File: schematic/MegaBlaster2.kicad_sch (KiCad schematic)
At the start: 119 parts, among them J1 USB_B, J2 SWD, J3 Micro_SD_Card, J4 AudioJack3, J5 DAC_Enable, SW2 SW_Push_Dual, SW3 SW_Push_Dual, SW4 SW_Push_Dual, SW5 SW_Push_Dual, SW6 SW_Push_Dual, SW7 SW_Push_Dual, U1 ATSAMD51J19A-A, U10 TPA6111A2DR, U11 YM2151, U2 LM2733XMF, U3 LD1117S33TR_SOT223, U4 LD1117S50TR_SOT223, U5 W25Q32JVSS, U6 Si5351A-B-GT, U7 TL074, U8 YM3012, U9 MCP6004, Y1 32.768KHz, Y2 25MHz

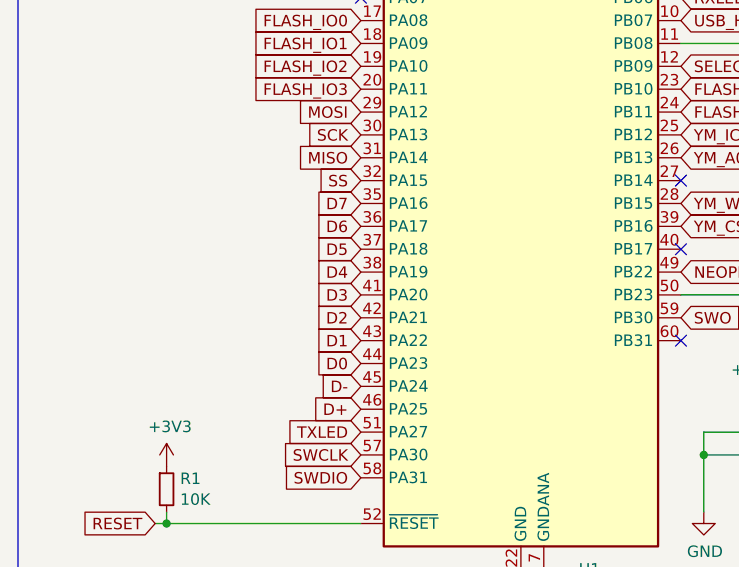
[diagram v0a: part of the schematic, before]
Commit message: PCB first pass
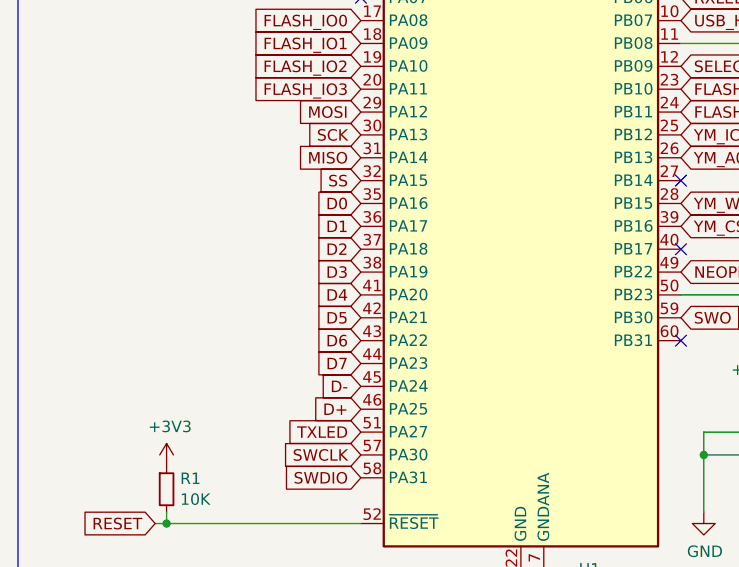
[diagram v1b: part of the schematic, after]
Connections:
- net D0: now also U1.35 (PA16); no longer U1.44 (PA23)
- net D1: now also U1.36 (PA17); no longer U1.43 (PA22)
- net D2: now also U1.37 (PA18); no longer U1.42 (PA21)
- net D3: now also U1.38 (PA19); no longer U1.41 (PA20)
- net D4: now also U1.41 (PA20); no longer U1.38 (PA19)
- net D5: now also U1.42 (PA21); no longer U1.37 (PA18)
- net D6: now also U1.43 (PA22); no longer U1.36 (PA17)
- net D7: now also U1.44 (PA23); no longer U1.35 (PA16)
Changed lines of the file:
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@@
     (effects (font (size 1.27 1.27)) (justify left bottom))
   )
-  (global_label "D7" (shape input) (at 52.07 87.63 180) (fields_autoplaced)
-    (effects (font (size 1.27 1.27)) (justify right))
-    (property "Intersheet References" "${INTERSHEET_REFS}" (id 0) (at 0 0 0)
+  (global_label "D7" (shape input) (at 52.07 105.41 180) (fields_autoplaced)
+    (effects (font (size 1.27 1.27)) (justify right))
+    (property "Intersheet References" "${INTERSHEET_REFS}" (id 0) (at 0 193.04 0)
       (effects (font (size 1.27 1.27)) hide)
     )
@@
     )
   )
-  (global_label "D4" (shape input) (at 52.07 95.25 180) (fields_autoplaced)
-    (effects (font (size 1.27 1.27)) (justify right))
-    (property "Intersheet References" "${INTERSHEET_REFS}" (id 0) (at 0 0 0)
+  (global_label "D4" (shape input) (at 52.07 97.79 180) (fields_autoplaced)
+    (effects (font (size 1.27 1.27)) (justify right))
+    (property "Intersheet References" "${INTERSHEET_REFS}" (id 0) (at 0 193.04 0)
       (effects (font (size 1.27 1.27)) hide)
     )
@@
     )
   )
-  (global_label "D2" (shape input) (at 52.07 100.33 180) (fields_autoplaced)
-    (effects (font (size 1.27 1.27)) (justify right))
-    (property "Intersheet References" "${INTERSHEET_REFS}" (id 0) (at 0 0 0)
+  (global_label "D2" (shape input) (at 52.07 92.71 180) (fields_autoplaced)
+    (effects (font (size 1.27 1.27)) (justify right))
+    (property "Intersheet References" "${INTERSHEET_REFS}" (id 0) (at 0 193.04 0)
       (effects (font (size 1.27 1.27)) hide)
     )
@@
     )
   )
-  (global_label "D5" (shape input) (at 52.07 92.71 180) (fields_autoplaced)
-    (effects (font (size 1.27 1.27)) (justify right))
-    (property "Intersheet References" "${INTERSHEET_REFS}" (id 0) (at 0 0 0)
+  (global_label "D5" (shape input) (at 52.07 100.33 180) (fields_autoplaced)
+    (effects (font (size 1.27 1.27)) (justify right))
+    (property "Intersheet References" "${INTERSHEET_REFS}" (id 0) (at 0 193.04 0)
       (effects (font (size 1.27 1.27)) hide)
     )
@@
     )
   )
-  (global_label "D3" (shape input) (at 52.07 97.79 180) (fields_autoplaced)
-    (effects (font (size 1.27 1.27)) (justify right))
-    (property "Intersheet References" "${INTERSHEET_REFS}" (id 0) (at 0 0 0)
+  (global_label "D3" (shape input) (at 52.07 95.25 180) (fields_autoplaced)
+    (effects (font (size 1.27 1.27)) (justify right))
+    (property "Intersheet References" "${INTERSHEET_REFS}" (id 0) (at 0 193.04 0)
       (effects (font (size 1.27 1.27)) hide)
     )
@@
     )
   )
-  (global_label "D6" (shape input) (at 52.07 90.17 180) (fields_autoplaced)
-    (effects (font (size 1.27 1.27)) (justify right))
-    (property "Intersheet References" "${INTERSHEET_REFS}" (id 0) (at 0 0 0)
-      (effects (font (size 1.27 1.27)) hide)
-    )
-  )
-  (global_label "D0" (shape input) (at 52.07 105.41 180) (fields_autoplaced)
-    (effects (font (size 1.27 1.27)) (justify right))
-    (property "Intersheet References" "${INTERSHEET_REFS}" (id 0) (at 0 0 0)
+  (global_label "D6" (shape input) (at 52.07 102.87 180) (fields_autoplaced)
+    (effects (font (size 1.27 1.27)) (justify right))
+    (property "Intersheet References" "${INTERSHEET_REFS}" (id 0) (at 0 193.04 0)
+      (effects (font (size 1.27 1.27)) hide)
+    )
+  )
+  (global_label "D0" (shape input) (at 52.07 87.63 180) (fields_autoplaced)
+    (effects (font (size 1.27 1.27)) (justify right))
+    (property "Intersheet References" "${INTERSHEET_REFS}" (id 0) (at 0 193.04 0)
       (effects (font (size 1.27 1.27)) hide)
     )
@@
     )
   )
-  (global_label "D1" (shape input) (at 52.07 102.87 180) (fields_autoplaced)
-    (effects (font (size 1.27 1.27)) (justify right))
-    (property "Intersheet References" "${INTERSHEET_REFS}" (id 0) (at 0 0 0)
-      (effects (font (size 1.27 1.27)) hide)
-    )
+  (global_label "D1" (shape input) (at 52.07 90.17 180) (fields_autoplaced)
+    (effects (font (size 1.27 1.27)) (justify right))
+    (property "Intersheet References" "${INTERSHEET_REFS}" (id 0) (at 0 193.04 0)
+      (effects (font (size 1.27 1.27)) hide)
+    )
